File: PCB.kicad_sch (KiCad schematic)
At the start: 69 parts, among them J1 USB_C_Receptacle_USB2.0_16P, J10 Conn_01x03_Pin, J2 Conn_01x03_Pin, J3 USB_C_Receptacle_USB2.0_16P, J4 Conn_01x08_Socket, J5 Conn_01x02_Pin, J6 Conn_01x04_Pin, J7 Conn_01x07_Pin, J9 Conn_01x03_Pin, Q1 S8050, Q2 S8050, SW1 SW_Push, SW2 SW_Push, SW3 SW_Push, SW4 SW_Push, SW5 SW_Push, SW6 RotaryEncoder_Switch_MP, U1 CH340C, U2 USBLC6-2SC6, U3 USBLC6-2SC6, U4 AMS1117-3.3 (UMW), U6 ESP32-S3-WROOM-1

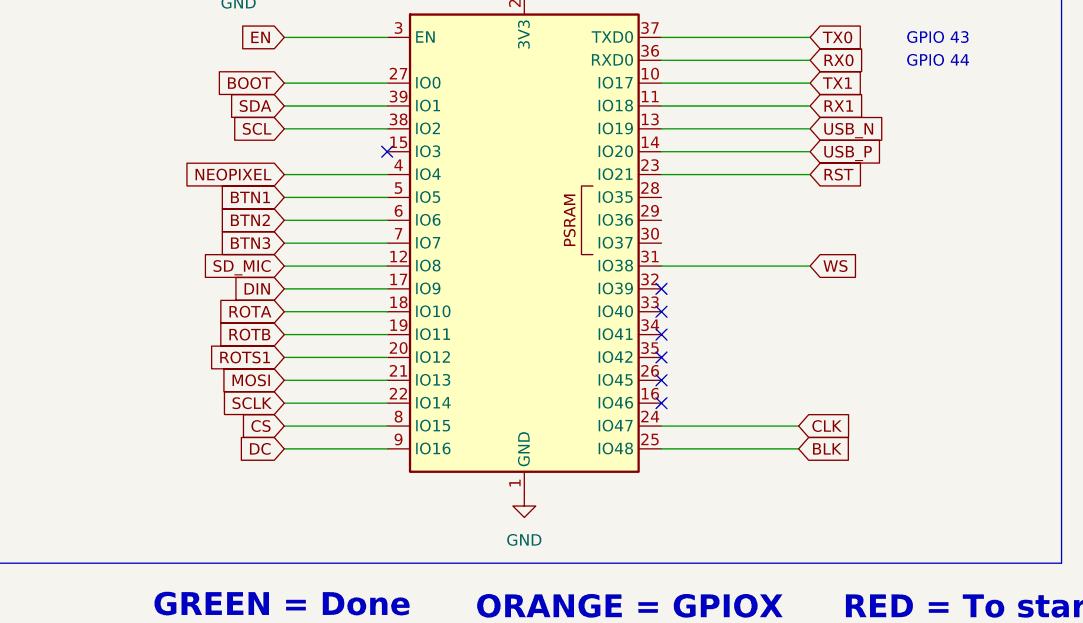
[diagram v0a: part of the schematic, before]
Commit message: fin routage
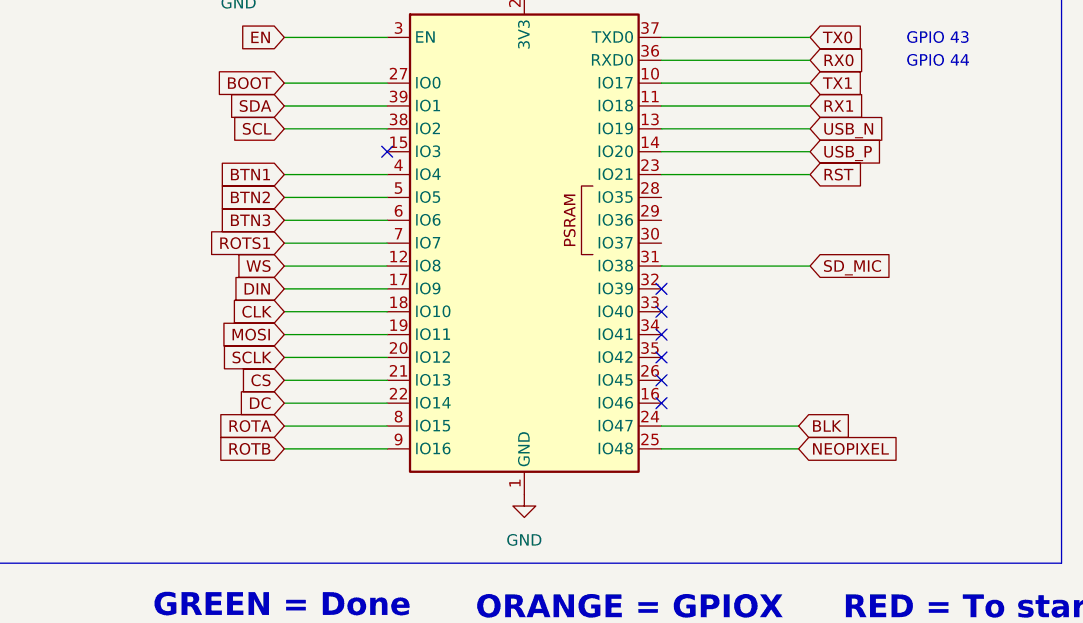
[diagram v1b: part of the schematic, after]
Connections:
- net BLK: now also U6.24 (IO47); no longer U6.25 (IO48)
- net BTN1: now also U6.4 (IO4); no longer U6.5 (IO5)
- net BTN2: now also U6.5 (IO5); no longer U6.6 (IO6)
- net BTN3: now also U6.6 (IO6); no longer U6.7 (IO7)
- net CLK: now also U6.18 (IO10); no longer U6.24 (IO47)
- net CS: now also U6.21 (IO13); no longer U6.8 (IO15)
- net DC: now also U6.22 (IO14); no longer U6.9 (IO16)
- net MOSI: now also U6.19 (IO11); no longer U6.21 (IO13)
- net NEOPIXEL: now also U6.25 (IO48); no longer U6.4 (IO4)
- net ROTA: now also U6.8 (IO15); no longer U6.18 (IO10)
- net ROTB: now also U6.9 (IO16); no longer U6.19 (IO11)
- net ROTS1: now also U6.7 (IO7); no longer U6.20 (IO12)
- net SCLK: now also U6.20 (IO12); no longer U6.22 (IO14)
- net SD_MIC: now also U6.31 (IO38); no longer U6.12 (IO8)
- net WS: now also U6.12 (IO8); no longer U6.31 (IO38)

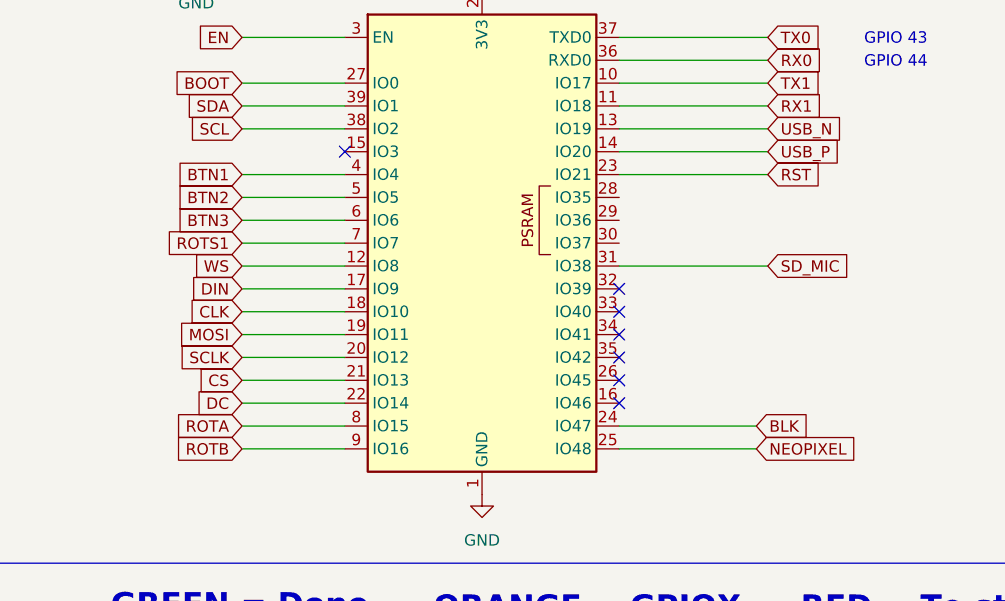
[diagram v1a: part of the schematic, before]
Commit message: test DRC
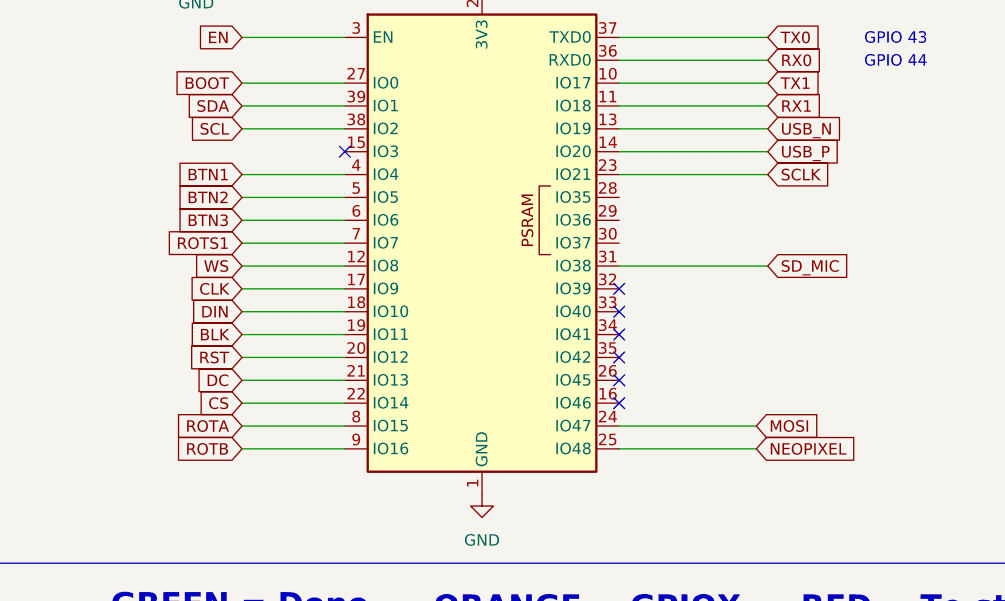
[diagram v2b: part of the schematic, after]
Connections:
- net BLK: now also U6.19 (IO11); no longer U6.24 (IO47)
- net CLK: now also U6.17 (IO9); no longer U6.18 (IO10)
- net CS: now also U6.22 (IO14); no longer U6.21 (IO13)
- net DC: now also U6.21 (IO13); no longer U6.22 (IO14)
- net DIN: now also U6.18 (IO10); no longer U6.17 (IO9)
- net MOSI: now also U6.24 (IO47); no longer U6.19 (IO11)
- net RST: now also U6.20 (IO12); no longer U6.23 (IO21)
- net SCLK: now also U6.23 (IO21); no longer U6.20 (IO12)
